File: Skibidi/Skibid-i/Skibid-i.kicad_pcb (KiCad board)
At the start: 2 copper layers, 140 x 78.5 mm, 61 parts, among them IC1 TEENSY_4.1, J1 Conn_01x02_Pin, J10 Screw_Terminal_01x03, J12 Screw_Terminal_01x03, J13 P78E05-1000, J14 Conn_01x02_Pin, J15 Conn_01x03_Pin, J16 Conn_01x02_Pin, J17 Conn_01x08_Pin, J18 Conn_01x02_Pin, J19 Conn_01x02_Pin, J2 Screw_Terminal_01x03, J20 Screw_Terminal_01x03, J21 Motor1, J22 Motor2, J3 Screw_Terminal_01x03, J4 Screw_Terminal_01x03, J5 Screw_Terminal_01x03, J6 Screw_Terminal_01x03, J7 Screw_Terminal_01x03, J8 Screw_Terminal_01x03, J9 Screw_Terminal_01x03, Q1 WL-OCPT_SERIES_357, Q2 WL-OCPT_SERIES_357, Q3 WL-OCPT_SERIES_357, Q4 WL-OCPT_SERIES_357, Q5 WL-OCPT_SERIES_357, Q6 WL-OCPT_SERIES_357, Q7 WL-OCPT_SERIES_357, SW2 210-4MS

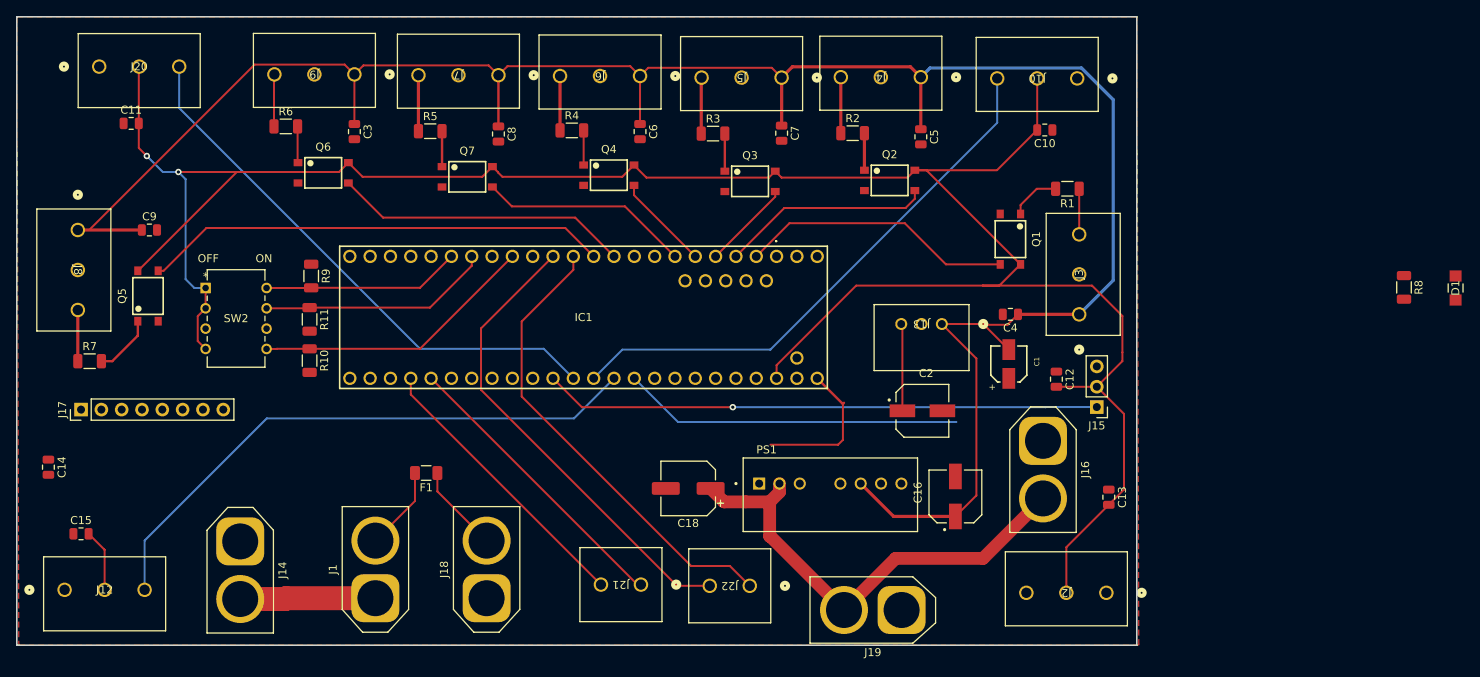
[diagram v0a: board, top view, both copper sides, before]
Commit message: ig im done
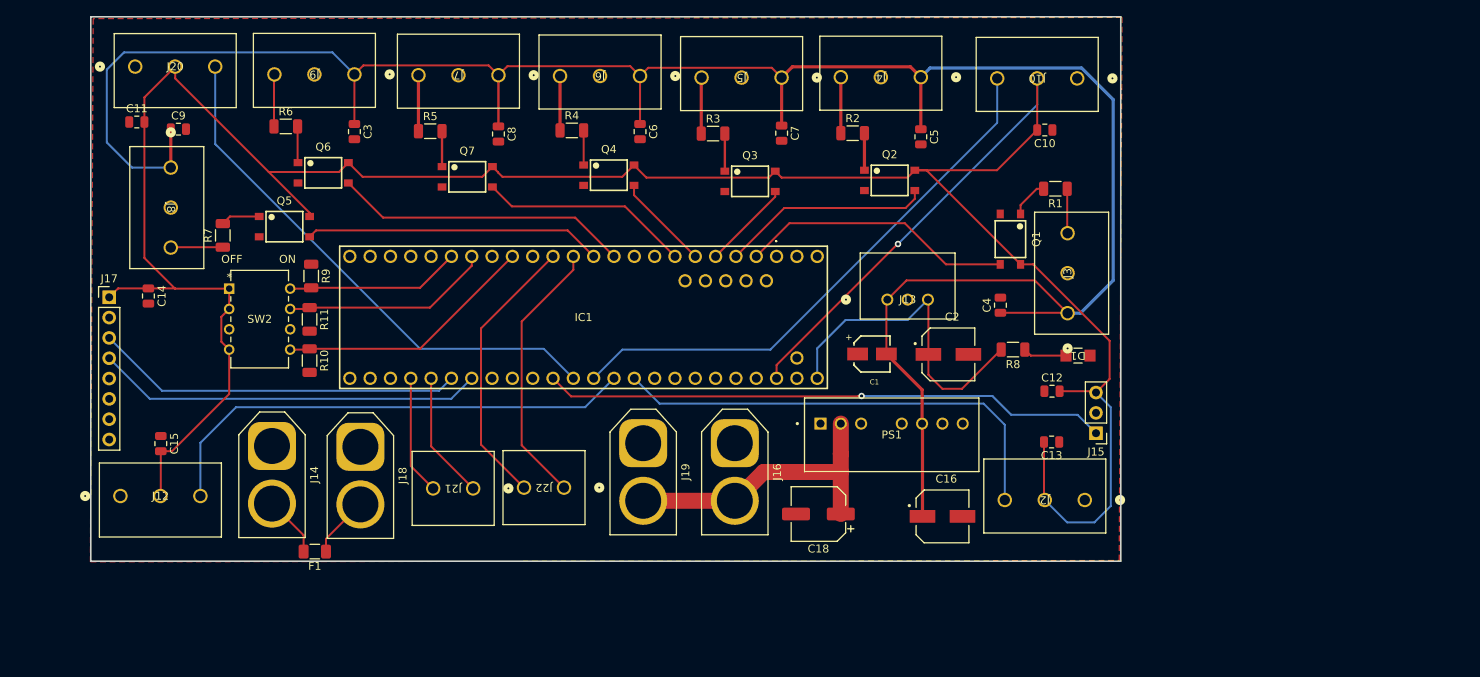
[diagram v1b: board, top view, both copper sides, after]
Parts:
- removed J1: Conn_01x02_Pin, Connector_AMASS:AMASS_XT60-F_1x02_P7.20mm_Vertical
- moved R8 49.5 mm to (259.0, 71.1), turned to 180 degrees
- moved D1 48.0 mm to (267.1, 71.8), turned to 180 degrees
- moved J16 38.5 mm to (224.2, 82.8)
- moved J19 38.4 mm to (212.8, 82.8), turned to -90 degrees
- moved J22 26.3 mm to (202.9, 88.3)
- moved C14 24.8 mm to (150.9, 64.4)
- moved J18 24.6 mm to (177.4, 83.2), turned to -90 degrees
- moved J21 24.2 mm to (191.5, 88.4)
- moved R7 22.9 mm to (160.2, 56.8), turned to 90 degrees
- moved Q5 19.1 mm to (167.9, 55.7), turned to 0 degrees
- moved C1 17.1 mm to (241.4, 71.7), turned to 180 degrees
- moved F1 17.0 mm to (171.8, 96.3)
- moved C18 16.6 mm to (234.7, 91.7)
- moved C15 15.1 mm to (152.5, 82.8), turned to -90 degrees
- moved J17 14.5 mm to (146.1, 64.6), turned to 0 degrees
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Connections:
- F1 pad 2: Net-(J1-Pin_2) -> Net-(J14-Pin_2)
- J14 pad 2: Net-(J1-Pin_1) -> Net-(J14-Pin_2)
- J15 pad 2: +3.3V -> GND
- J15 pad 3: GND -> +3.3V
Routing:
- net SDA: track 0.00 -> 48.5 mm
- net SCL: track 0.00 -> 46.2 mm
- net +3.3V: track 307.2 -> 340.7 mm, vias 2 -> 1
- net BDC1: track 58.5 -> 33.8 mm
- net BDC11: track 59.1 -> 34.9 mm
- net +48V: track 58.9 -> 37.5 mm
- net BDC2: track 36.9 -> 15.9 mm
- net Dis7: track 58.1 -> 37.2 mm
- net BDC22: track 35.6 -> 14.9 mm
- net Net-(J1-Pin_1): track 17.0 -> 0.00 mm
- net LN4: track 42.5 -> 58.1 mm
- net Net-(J1-Pin_2): track 11.9 -> 0.00 mm
- net +5V: track 29.6 -> 41.4 mm
- net LN3: track 73.2 -> 61.7 mm
- net Net-(J14-Pin_2): track 0.00 -> 7.64 mm
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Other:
- board size 140 x 78.5 mm -> 128.7 x 68 mm

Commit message: erm what the sigma
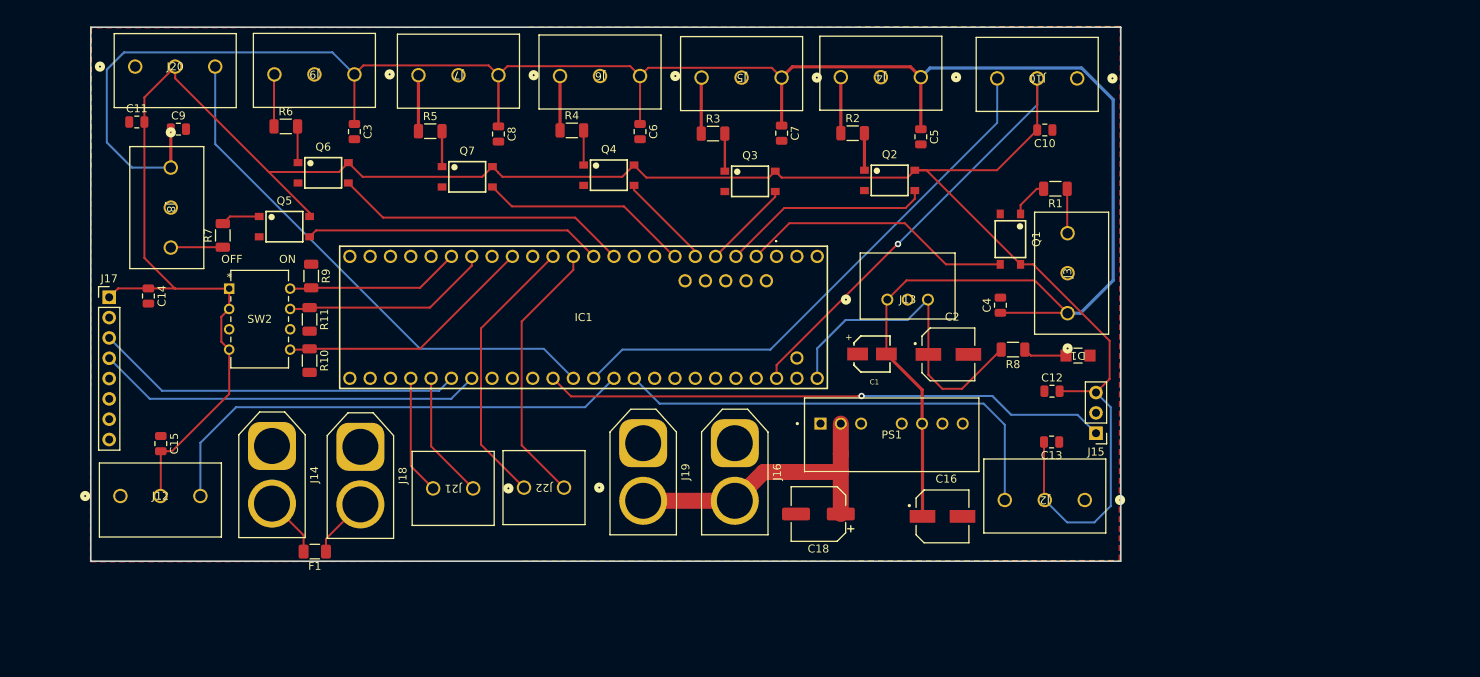
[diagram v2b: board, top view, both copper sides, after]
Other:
- board size 128.7 x 68 mm -> 128.7 x 66.8 mm
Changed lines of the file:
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@@
 		(at 243.8625 81.75)
 		(property "Reference" "PS1"
-			(at 0 0 360)
+			(at 0 0 0)
 			(layer "F.SilkS")
 			(effects
@@
 		)
 		(property "Value" "RSO-4812S_H2"
-			(at -0.355 5.665 360)
+			(at -0.355 5.665 0)
 			(layer "F.Fab")
 			(effects
@@
 		)
 		(property "Footprint" "askibidi:12vConvertor"
-			(at 0 0 360)
+			(at 0 0 0)
 			(layer "F.Fab")
 			(hide yes)
@@
 		)
 		(property "Datasheet" ""
-			(at 0 0 360)
+			(at 0 0 0)
 			(layer "F.Fab")
 			(hide yes)
@@
 		)
 		(property "Description" ""
-			(at 0 0 360)
+			(at 0 0 0)
 			(layer "F.Fab")
 			(hide yes)
@@
 		(tags "Through hole pin header THT 1x03 2.54mm single row")
 		(property "Reference" "J15"
-			(at 0 -2.33 360)
+			(at 0 -2.33 0)
 			(layer "F.SilkS")
 			(effects
@@
 		)
 		(property "Value" "Conn_01x03_Pin"
-			(at 0 7.41 360)
+			(at 0 7.41 0)
 			(layer "F.Fab")
 			(effects
@@
 		(tags "capacitor")
 		(property "Reference" "C13"
-			(at 0 -1.68 360)
+			(at 0 -1.68 0)
 			(layer "F.SilkS")
 			(effects
@@
 		)
 		(property "Value" "0.1uF"
-			(at 0 1.68 360)
+			(at 0 1.68 0)
 			(layer "F.Fab")
 			(effects
@@
 		)
 		(fp_text user "${REFERENCE}"
-			(at 0 0 360)
+			(at 0 0 0)
 			(layer "F.Fab")
 			(effects
@@
 		(tags "capacitor")
 		(property "Reference" "R8"
-			(at 0 -1.85 360)
+			(at 0 -1.85 0)
 			(layer "F.SilkS")
 			(effects
@@
 		)
 		(property "Value" "500ohm"
-			(at 0 1.85 360)
+			(at 0 1.85 0)
 			(layer "F.Fab")
 			(effects
@@
 		)
 		(fp_text user "${REFERENCE}"
-			(at 0 0 360)
+			(at 0 0 0)
 			(layer "F.Fab")
 			(effects
@@
 		)
 		(property "Footprint" "askibidi:5vregulator"
-			(at 0 0 360)
+			(at 0 0 0)
 			(layer "F.Fab")
 			(hide yes)
@@
 		)
 		(property "Datasheet" "P78E05-1000"
-			(at 0 0 360)
+			(at 0 0 0)
 			(layer "F.Fab")
 			(hide yes)
@@
 		)
 		(property "Description" ""
-			(at 0 0 360)
+			(at 0 0 0)
 			(layer "F.Fab")
 			(hide yes)
@@
 		)
 		(property "Footprint" "askibidi:LED"
-			(at 0 0 360)
+			(at 0 0 0)
 			(layer "F.Fab")
 			(hide yes)
@@
 		)
 		(property "Datasheet" ""
-			(at 0 0 360)
+			(at 0 0 0)
 			(layer "F.Fab")
 			(hide yes)
@@
 		)
 		(property "Description" "Light emitting diode"
-			(at 0 0 360)
+			(at 0 0 0)
 			(layer "F.Fab")
 			(hide yes)
@@
 		(tags "capacitor electrolytic")
 		(property "Reference" "C18"
-			(at 0 -4.35 360)
+			(at 0 -4.35 0)
 			(layer "F.SilkS")
 			(effects
@@
 		)
 		(property "Value" "100uF"
-			(at 0 4.35 360)
+			(at 0 4.35 0)
 			(layer "F.Fab")
 			(effects
@@
 		)
 		(fp_text user "${REFERENCE}"
-			(at 0 0 360)
+			(at 0 0 0)
 			(layer "F.Fab")
 			(effects
@@
 		(descr "<b> WL-OCPT Optocoupler Phototransistor</b><br>Size : SOP4, SMT, 4pins")
 		(property "Reference" "Q5"
-			(at 0 -3.235 360)
+			(at 0 -3.235 0)
 			(layer "F.SilkS")
 			(effects
@@
 		)
 		(property "Value" "WL-OCPT_SERIES_357"
-			(at 0.05 -4.8899 360)
+			(at 0.05 -4.8899 0)
 			(layer "F.Fab")
 			(effects
@@
 		)
 		(property "Footprint" "askibidi:optopt"
-			(at 0 0 360)
+			(at 0 0 0)
 			(layer "F.Fab")
 			(hide yes)
@@
 		)
 		(property "Datasheet" ""
-			(at 0 0 360)
+			(at 0 0 0)
 			(layer "F.Fab")
 			(hide yes)
@@
 		)
 		(property "Description" ""
-			(at 0 0 360)
+			(at 0 0 0)
 			(layer "F.Fab")
 			(hide yes)
@@
 		(descr "<B>WCAP-ASLI</B><BR> Aluminium Electrolytic Capacitors,4X5.5X1(DiameterXLengthXPitch)")
 		(property "Reference" "C1"
-			(at -0.3 -3.5064 360)
+			(at -0.3 -3.5064 0)
 			(layer "F.SilkS")
 			(effects
@@
 		)
 		(property "Value" "10uF"
-			(at -0.5 3.4936 360)
+			(at -0.5 3.4936 0)
 			(layer "F.Fab")
 			(effects
@@
 		)
 		(property "Footprint" "askibidi:10uF"
-			(at 0 0 360)
+			(at 0 0 0)
 			(layer "F.Fab")
 			(hide yes)
@@
 		)
 		(property "Datasheet" ""
-			(at 0 0 360)
+			(at 0 0 0)
 			(layer "F.Fab")
 			(hide yes)
@@
 		)
 		(property "Description" "Unpolarized capacitor"
-			(at 0 0 360)
+			(at 0 0 0)
 			(layer "F.Fab")
 			(hide yes)
@@
 		)
 		(fp_text user "+"
-			(at 2.9 2.1 360)
+			(at 2.9 2.1 0)
 			(layer "F.SilkS")
 			(effects
@@
 		(tags "capacitor")
 		(property "Reference" "C12"
-			(at 0 -1.68 360)
+			(at 0 -1.68 0)
 			(layer "F.SilkS")
 			(effects
@@
 		)
 		(property "Value" "0.1uF"
-			(at 0 1.68 360)
+			(at 0 1.68 0)
 			(layer "F.Fab")
 			(effects
@@
 		)
 		(fp_text user "${REFERENCE}"
-			(at 0 0 360)
+			(at 0 0 0)
 			(layer "F.Fab")
 			(effects
@@
 		(tags "fuse")
 		(property "Reference" "F1"
-			(at 0 -1.82 360)
+			(at 0 -1.82 0)
 			(layer "F.SilkS")
 			(effects
@@
 		)
 		(property "Value" "Fuse"
-			(at 0 1.82 360)
+			(at 0 1.82 0)
 			(layer "F.Fab")
 			(effects
@@
 		)
 		(fp_text user "${REFERENCE}"
-			(at 0 0 360)
+			(at 0 0 0)
 			(layer "F.Fab")
 			(effects
@@
 		(tags "Through hole pin header THT 1x08 2.54mm single row")
 		(property "Reference" "J17"
-			(at 0 -2.33 360)
+			(at 0 -2.33 0)
 			(layer "F.SilkS")
 			(effects
@@
 		)
 		(property "Value" "Conn_01x08_Pin"
-			(at -0.08 23.06 360)
+			(at -0.08 23.06 0)
 			(layer "F.Fab")
 			(effects
@@
 		(at 250.95 71.7)
 		(property "Reference" "C2"
-			(at 0.475 -4.685 360)
+			(at 0.475 -4.685 0)
 			(layer "F.SilkS")
 			(effects
@@
 		)
 		(property "Value" "22uF"
-			(at 0.35 2.05 360)
+			(at 0.35 2.05 0)
 			(layer "F.Fab")
 			(effects
@@
 		)
 		(property "Footprint" "askibidi:Ecap"
-			(at 0 0 360)
+			(at 0 0 0)
 			(layer "F.Fab")
 			(hide yes)
@@
 		)
 		(property "Datasheet" ""
-			(at 0 0 360)
+			(at 0 0 0)
 			(layer "F.Fab")
 			(hide yes)
@@
 		)
 		(property "Description" "Unpolarized capacitor"
-			(at 0 0 360)
+			(at 0 0 0)
 			(layer "F.Fab")
 			(hide yes)
@@
 		(at 250.2125 91.95)
 		(property "Reference" "C16"
-			(at 0.475 -4.685 360)
+			(at 0.475 -4.685 0)
 			(layer "F.SilkS")
 			(effects
@@
 		)
 		(property "Value" "22uF"
-			(at 4.1 -4.85 360)
+			(at 4.1 -4.85 0)
 			(layer "F.Fab")
 			(effects
@@
 		)
 		(property "Footprint" "askibidi:Ecap"
-			(at 0 0 360)
+			(at 0 0 0)
 			(layer "F.Fab")
 			(hide yes)
@@
 		)
 		(property "Datasheet" ""
-			(at 0 0 360)
+			(at 0 0 0)
 			(layer "F.Fab")
 			(hide yes)
@@
 		)
 		(property "Description" "Polarized capacitor, US symbol"
-			(at 0 0 360)
+			(at 0 0 0)
 			(layer "F.Fab")
 			(hide yes)
@@
 	)
 	(gr_rect
-		(start 143.75 29.5)
+		(start 143.75 30.8)
 		(end 272.496 97.55)
 		(stroke
@@
 	)
 	(segment
-		(start 211.654899 51.794899)
-		(end 219.31 59.45)
+		(start 211.654899 50.57)
+		(end 211.654899 51.154899)
 		(width 0.25)
 		(layer "F.Cu")
@@
 	)
 	(segment
-		(start 211.654899 50.57)
-		(end 211.654899 51.794899)
+		(start 211.654899 51.154899)
+		(end 219.31 58.81)
 		(width 0.25)
 		(layer "F.Cu")
@@
 	)
 	(segment
+		(start 219.31 58.81)
+		(end 219.31 59.45)
+		(width 0.25)
+		(layer "F.Cu")
+		(net 46)
+	)
+	(segment
 		(start 250.645101 60.445101)
 		(end 257.43 60.445101)
@@
 	)
 	(segment
-		(start 210.52 53.2)
-		(end 216.77 59.45)
+		(start 193.954899 50.77)
+		(end 196.384899 53.2)
+		(width 0.25)
+		(layer "F.Cu")
+		(net 59)
+	)
+	(segment
+		(start 210.4 53.2)
+		(end 216.65 59.45)
 		(width 0.25)
 		(layer "F.Cu")
@@
 	(segment
 		(start 196.384899 53.2)
-		(end 210.52 53.2)
+		(end 210.4 53.2)
 		(width 0.25)
 		(layer "F.Cu")
@@
 	)
 	(segment
-		(start 193.954899 50.77)
-		(end 196.384899 53.2)
+		(start 216.65 59.45)
+		(end 216.77 59.45)
 		(width 0.25)
 		(layer "F.Cu")
@@
 		(polygon
 			(pts
-				(xy 144.05 29.725) (xy 143.7 97.625) (xy 272.304 97.470101) (xy 272.654 29.570101)
+				(xy 143.823 30.875) (xy 143.7 97.625) (xy 272.304 97.470101) (xy 272.427 30.720101)
 			)
 		)
